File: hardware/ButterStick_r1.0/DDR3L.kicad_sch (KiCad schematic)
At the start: 14 parts, among them U12 MT41K64M16TW-107_J-TR

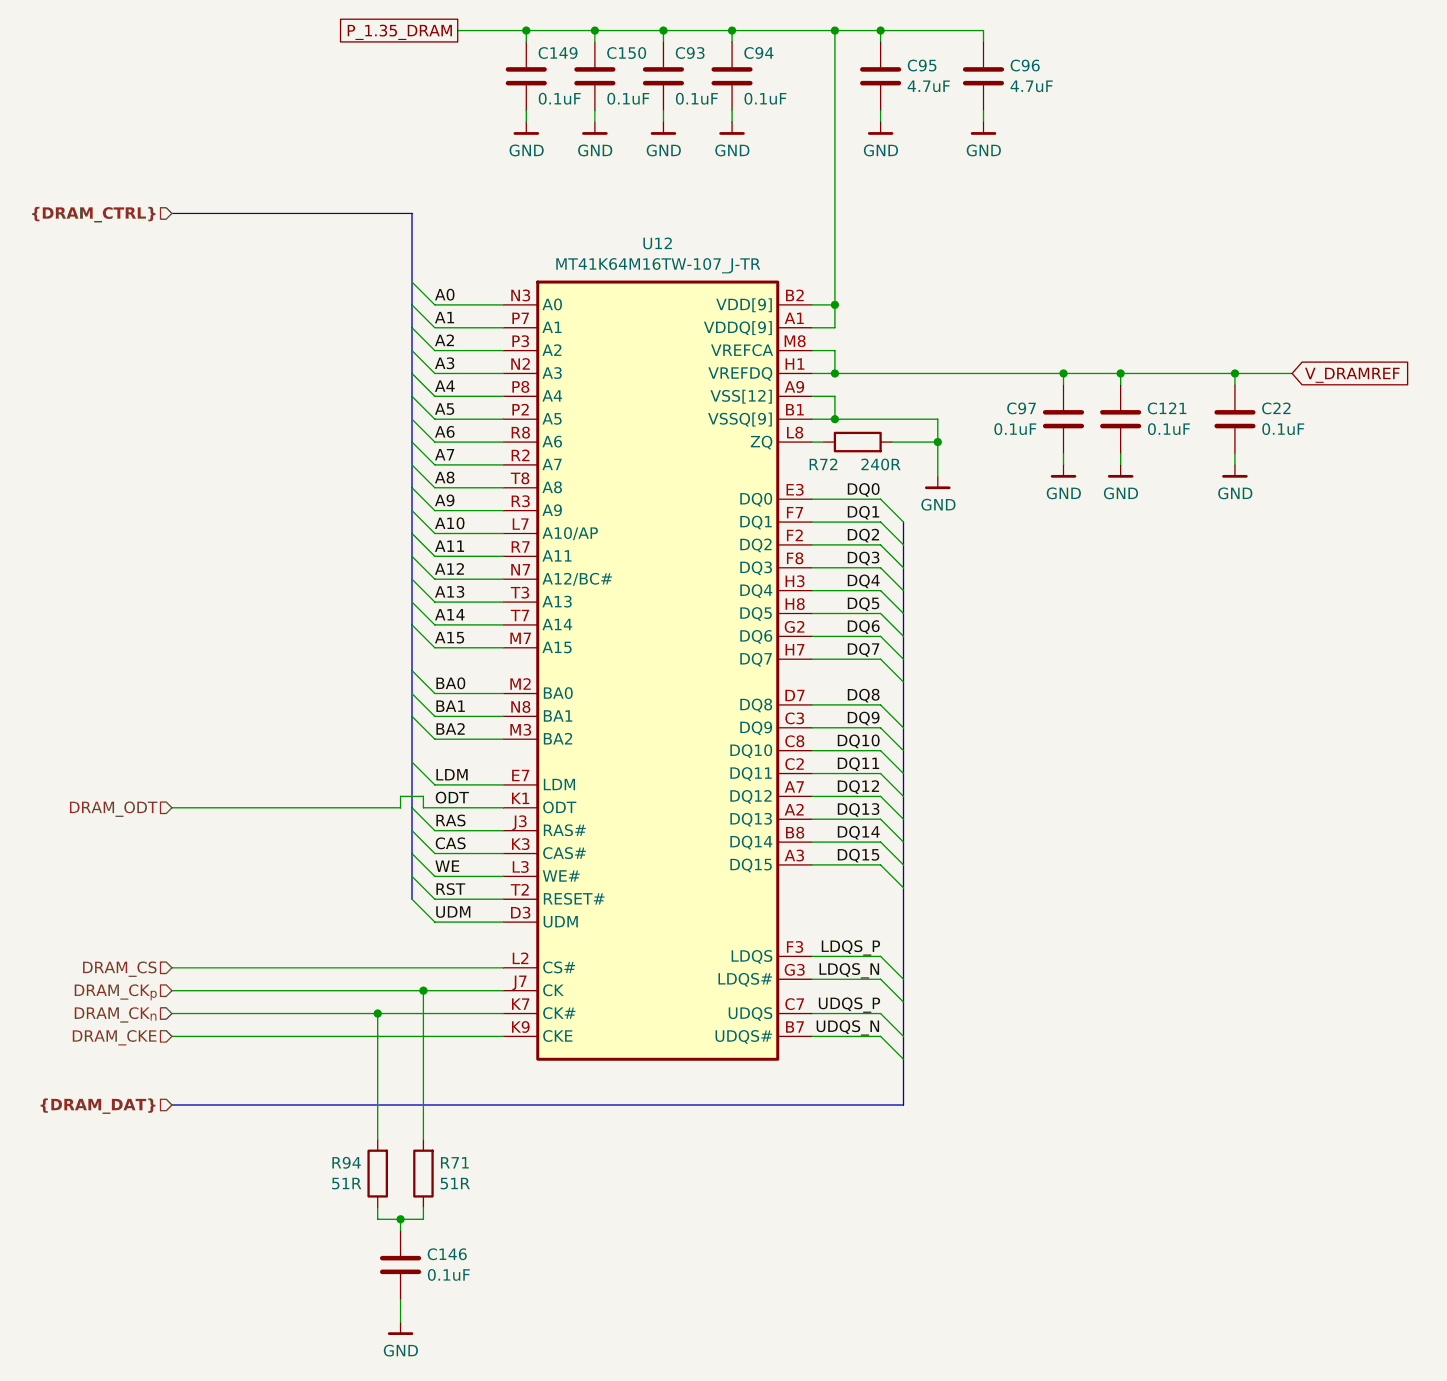
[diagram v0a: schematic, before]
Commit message: hw.r1d0: Review complete, gerbers generated
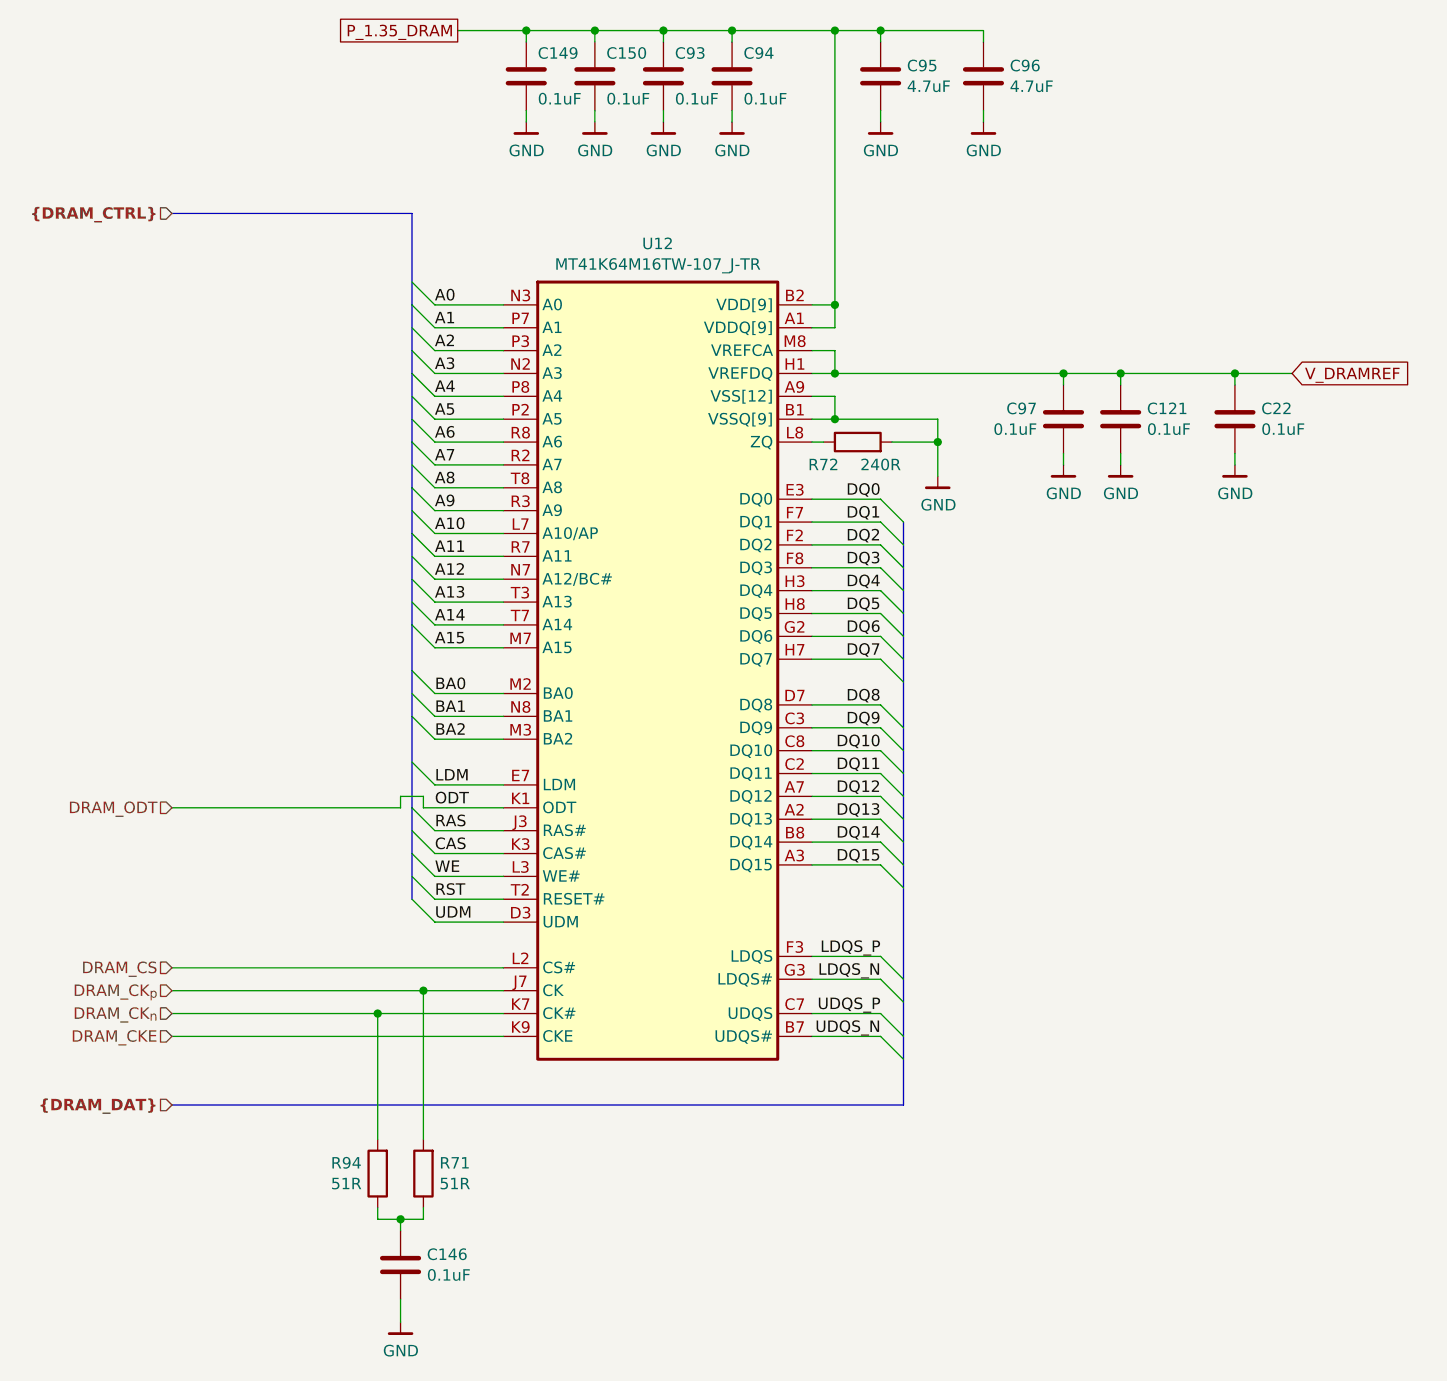
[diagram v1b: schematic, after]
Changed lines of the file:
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@@
   (title_block
     (title "ButterStick")
-    (date "2020-07-16")
+    (date "2020-07-17")
     (rev "r1.0")
     (company "GsD")
@@
     (stroke (width 0) (type solid) (color 0 0 0 0))
   )
-  (bus (pts (xy 110.49 66.04) (xy 110.49 68.58))
-    (stroke (width 0) (type solid) (color 0 0 0 0))
-  )
-  (bus (pts (xy 110.49 68.58) (xy 110.49 73.66))
-    (stroke (width 0) (type solid) (color 0 0 0 0))
-  )
-  (bus (pts (xy 110.49 73.66) (xy 110.49 76.2))
-    (stroke (width 0) (type solid) (color 0 0 0 0))
-  )
-  (bus (pts (xy 110.49 76.2) (xy 110.49 81.28))
+  (bus (pts (xy 110.49 66.04) (xy 110.49 71.12))
+    (stroke (width 0) (type solid) (color 0 0 0 0))
+  )
+  (bus (pts (xy 110.49 71.12) (xy 110.49 73.66))
+    (stroke (width 0) (type solid) (color 0 0 0 0))
+  )
+  (bus (pts (xy 110.49 73.66) (xy 110.49 78.74))
+    (stroke (width 0) (type solid) (color 0 0 0 0))
+  )
+  (bus (pts (xy 110.49 78.74) (xy 110.49 81.28))
     (stroke (width 0) (type solid) (color 0 0 0 0))
   )
@@
     (stroke (width 0) (type solid) (color 0 0 0 0))
   )
-  (bus (pts (xy 165.1 90.17) (xy 165.1 92.71))
-    (stroke (width 0) (type solid) (color 0 0 0 0))
-  )
-  (bus (pts (xy 165.1 92.71) (xy 165.1 97.79))
-    (stroke (width 0) (type solid) (color 0 0 0 0))
-  )
-  (bus (pts (xy 165.1 97.79) (xy 165.1 102.87))
-    (stroke (width 0) (type solid) (color 0 0 0 0))
-  )
-  (bus (pts (xy 165.1 102.87) (xy 165.1 105.41))
+  (bus (pts (xy 165.1 90.17) (xy 165.1 95.25))
+    (stroke (width 0) (type solid) (color 0 0 0 0))
+  )
+  (bus (pts (xy 165.1 95.25) (xy 165.1 100.33))
+    (stroke (width 0) (type solid) (color 0 0 0 0))
+  )
+  (bus (pts (xy 165.1 100.33) (xy 165.1 105.41))
     (stroke (width 0) (type solid) (color 0 0 0 0))
   )
@@
     (stroke (width 0) (type solid) (color 0 0 0 0))
   )
-  (bus (pts (xy 165.1 118.11) (xy 165.1 120.65))
-    (stroke (width 0) (type solid) (color 0 0 0 0))
-  )
-  (bus (pts (xy 165.1 120.65) (xy 165.1 125.73))
-    (stroke (width 0) (type solid) (color 0 0 0 0))
-  )
-  (bus (pts (xy 165.1 125.73) (xy 165.1 130.81))
-    (stroke (width 0) (type solid) (color 0 0 0 0))
-  )
-  (bus (pts (xy 165.1 130.81) (xy 165.1 143.51))
-    (stroke (width 0) (type solid) (color 0 0 0 0))
-  )
-  (bus (pts (xy 165.1 143.51) (xy 165.1 149.86))
-    (stroke (width 0) (type solid) (color 0 0 0 0))
-  )
-  (bus (pts (xy 165.1 149.86) (xy 165.1 154.94))
-    (stroke (width 0) (type solid) (color 0 0 0 0))
-  )
+  (bus (pts (xy 165.1 118.11) (xy 165.1 123.19))
+    (stroke (width 0) (type solid) (color 0 0 0 0))
+  )
+  (bus (pts (xy 165.1 123.19) (xy 165.1 128.27))
+    (stroke (width 0) (type solid) (color 0 0 0 0))
+  )
+  (bus (pts (xy 165.1 128.27) (xy 165.1 140.97))
+    (stroke (width 0) (type solid) (color 0 0 0 0))
+  )
+  (bus (pts (xy 165.1 140.97) (xy 165.1 147.32))
+    (stroke (width 0) (type solid) (color 0 0 0 0))
+  )
+  (bus (pts (xy 165.1 147.32) (xy 165.1 154.94))
+    (stroke (width 0) (type solid) (color 0 0 0 0))
+  )
